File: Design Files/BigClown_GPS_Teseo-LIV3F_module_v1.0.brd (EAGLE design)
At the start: 40.3 x 66 mm, 17 parts, among them IC1 TESEO-LIV3F, X1 SMA-SMD, X2 BU-SMA-H

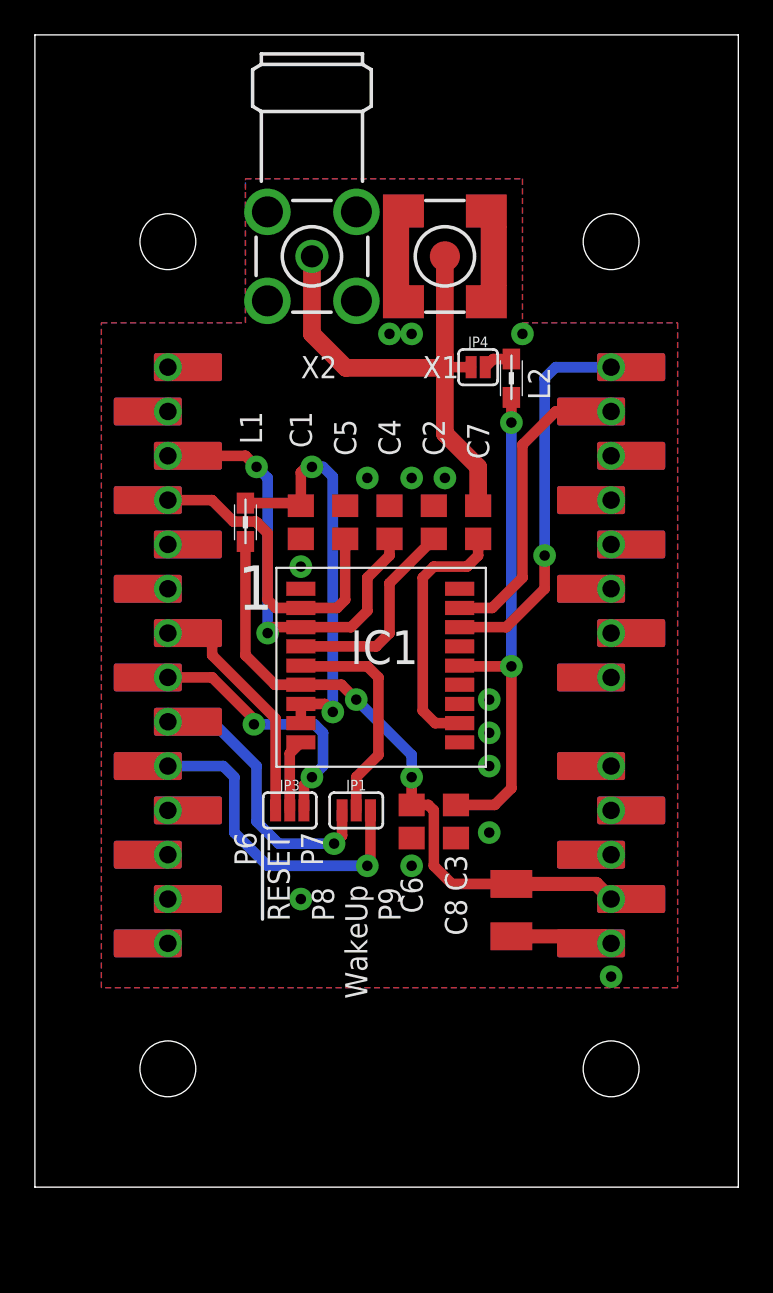
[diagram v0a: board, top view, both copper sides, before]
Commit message: Add files via upload
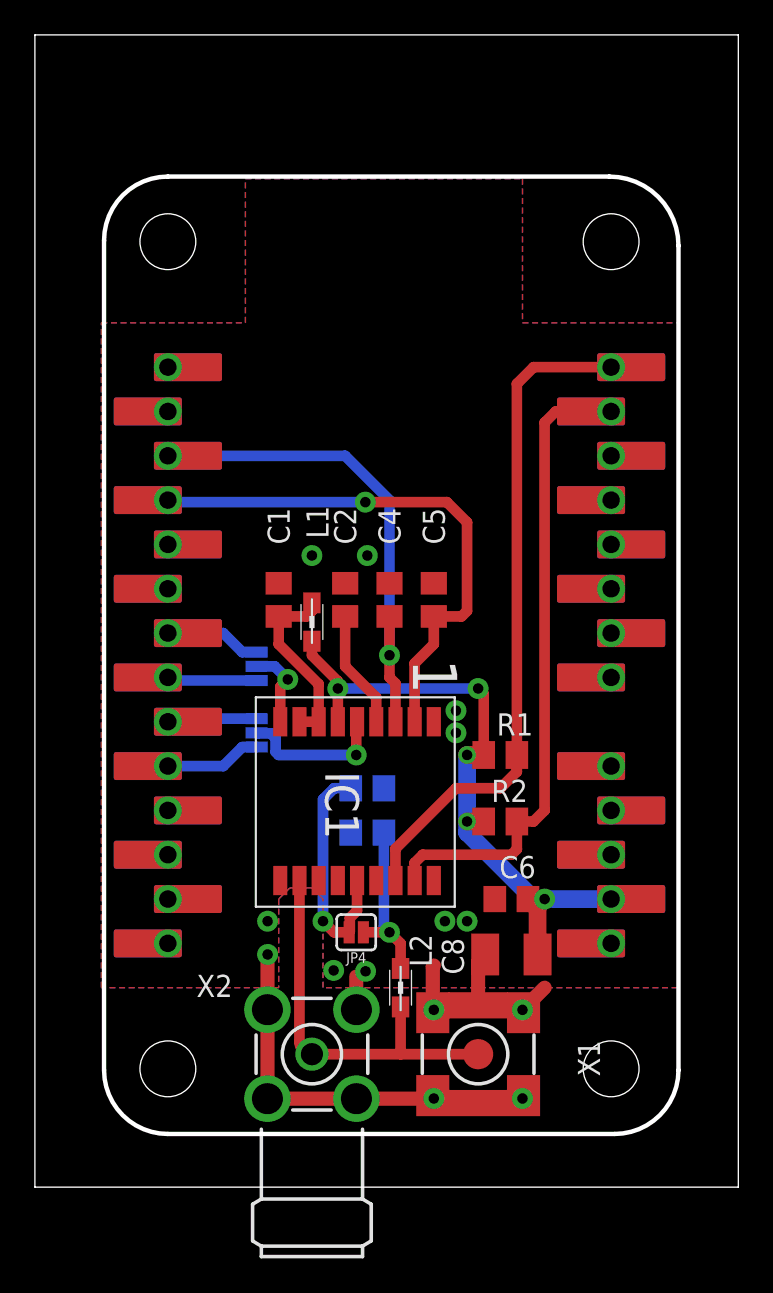
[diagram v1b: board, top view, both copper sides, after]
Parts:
- added R1, R2: (no value), rcl:M0805
- moved X1 45.8 mm to (25.4, 7.62), turned to 90 degrees
- moved X2 45.7 mm to (15.9, 7.62), turned to 270 degrees
- moved L2 35.5 mm to (21.0, 11.4), turned to 90 degrees
- moved JP4 33.1 mm to (18.4, 14.6), turned to 180 degrees
- moved C7 18.9 mm to (19.1, 20.3), flipped to the bottom, turned to 0 degrees
- moved IC1 10.8 mm to (22.9, 26.7), turned to 0 degrees
- moved JP3 8.47 mm to (12.7, 29.8), flipped to the bottom, turned to 270 degrees
- moved JP1 7.24 mm to (12.7, 26.0), flipped to the bottom, turned to 270 degrees
- moved C6 7.24 mm to (27.3, 16.5), turned to 180 degrees
- moved L1 6.87 mm to (15.9, 32.4)
- moved C2 6.75 mm to (17.8, 33.7)
- moved C5 6.75 mm to (22.9, 33.7)
- moved C3 5.43 mm to (19.1, 22.9), flipped to the bottom, turned to 180 degrees
- moved C1 4.62 mm to (14.0, 33.7), turned to 90 degrees
- moved C4 4.45 mm to (20.3, 33.7)
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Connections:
- removed net N$5: C7.2, IC1.11
- net GND: now also C7.2
- net N$2: now also IC1.11, L2.1; no longer C7.1, JP4.1
- net N$3: now also C7.1, JP4.1, L2.2; no longer JP4.2, L2.1
- net SCL: now also R2.1
- net SDA: now also R1.1
- net VCC: now also R1.2, R2.2
- net VCC_RF: now also JP4.2; no longer L2.2
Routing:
- net GND: track 5.88 -> 38.6 mm, vias 14 -> 10
- net SCL: track 17.8 -> 36.9 mm
- net SDA: track 21.9 -> 38.6 mm, vias 1 -> 0
- net VCC_RF: track 28.9 -> 13.8 mm, vias 2 -> 1
- net N$5: track 14.7 -> 0.00 mm
- net P9: track 18.9 -> 5.53 mm, vias 1 -> 0
- net N$1: track 23.9 -> 10.6 mm, vias 2 -> 0
- net RX: track 18.6 -> 31.3 mm, vias 0 -> 1
- net P8: track 16.4 -> 5.15 mm, vias 1 -> 0
- net P7: track 15.4 -> 5.15 mm, vias 2 -> 0
- net P6: track 14.2 -> 5.53 mm
- net N$3: track 1.69 -> 9.68 mm, vias 0 -> 1
- net N$2: track 29.5 -> 22.5 mm
- net PPS: track 11.8 -> 6.77 mm
- net WAKE_UP: track 12.9 -> 8.63 mm, vias 0 -> 1
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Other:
- outline, holes or cut-outs redrawn
- board text removed: "!RESET"
- board text removed: "P6"
- board text removed: "P7"
- board text removed: "P8"
- board text removed: "P9"
- board text removed: "WakeUp"
